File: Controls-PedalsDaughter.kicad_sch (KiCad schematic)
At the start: 3 parts, among them J3 PeripheralCANConnector, J5 PeripheralCANConnector, U2 PeripheralSOM

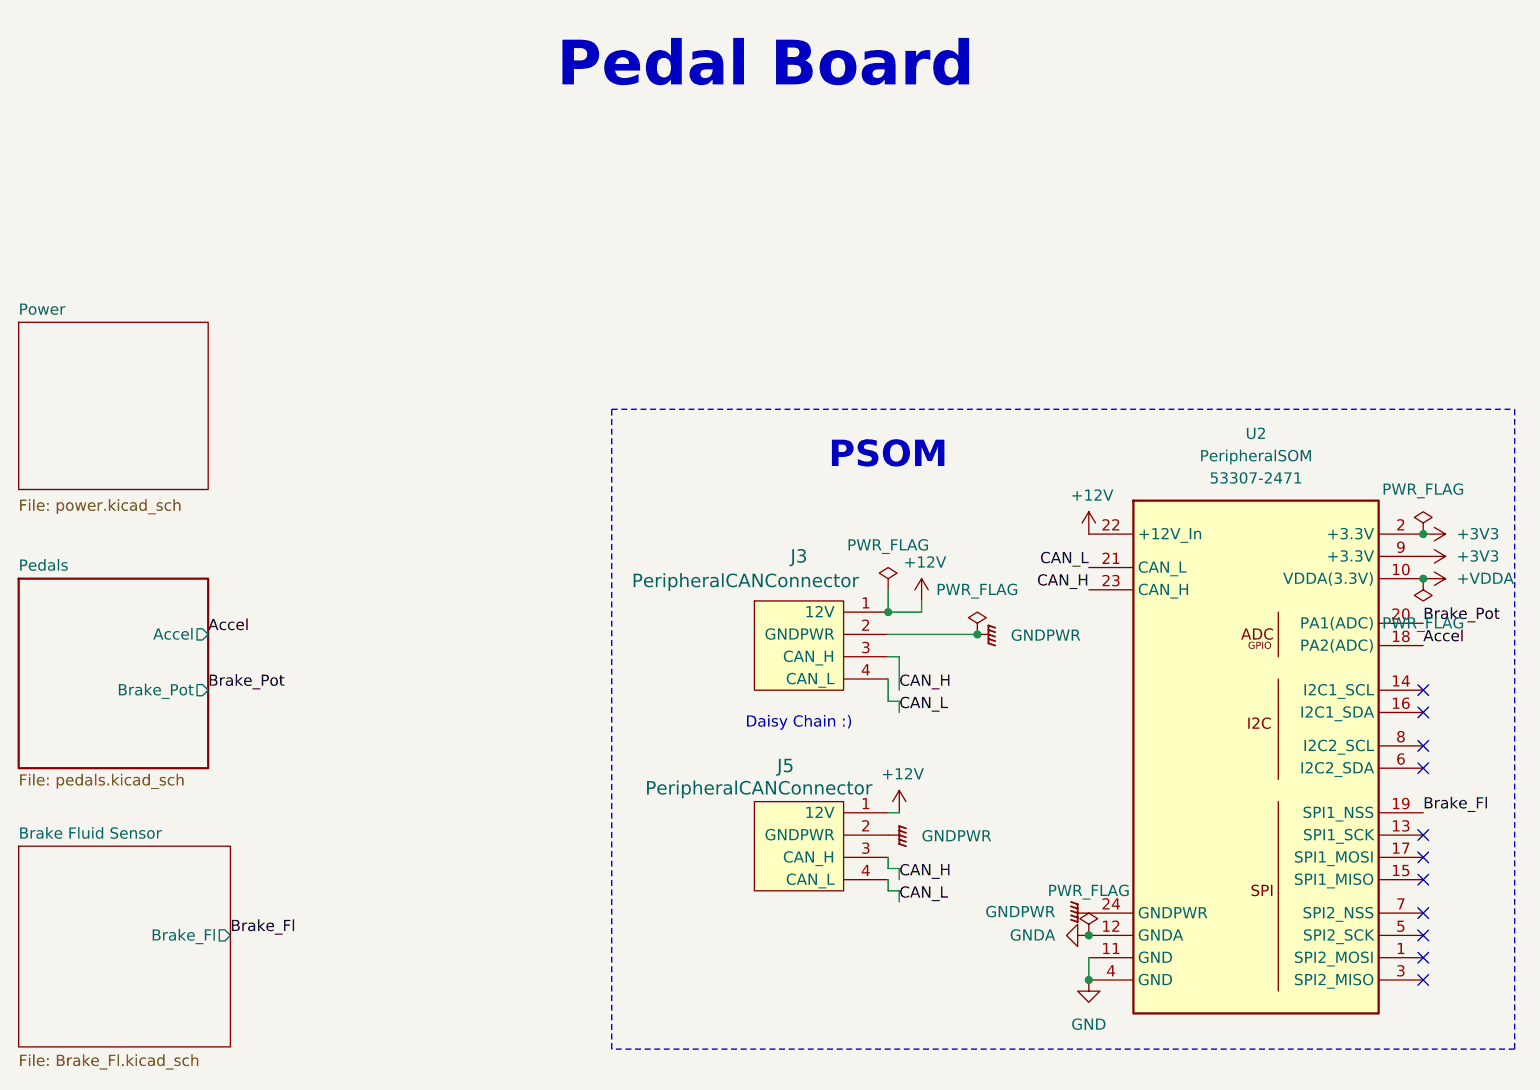
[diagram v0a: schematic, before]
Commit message: new constraints
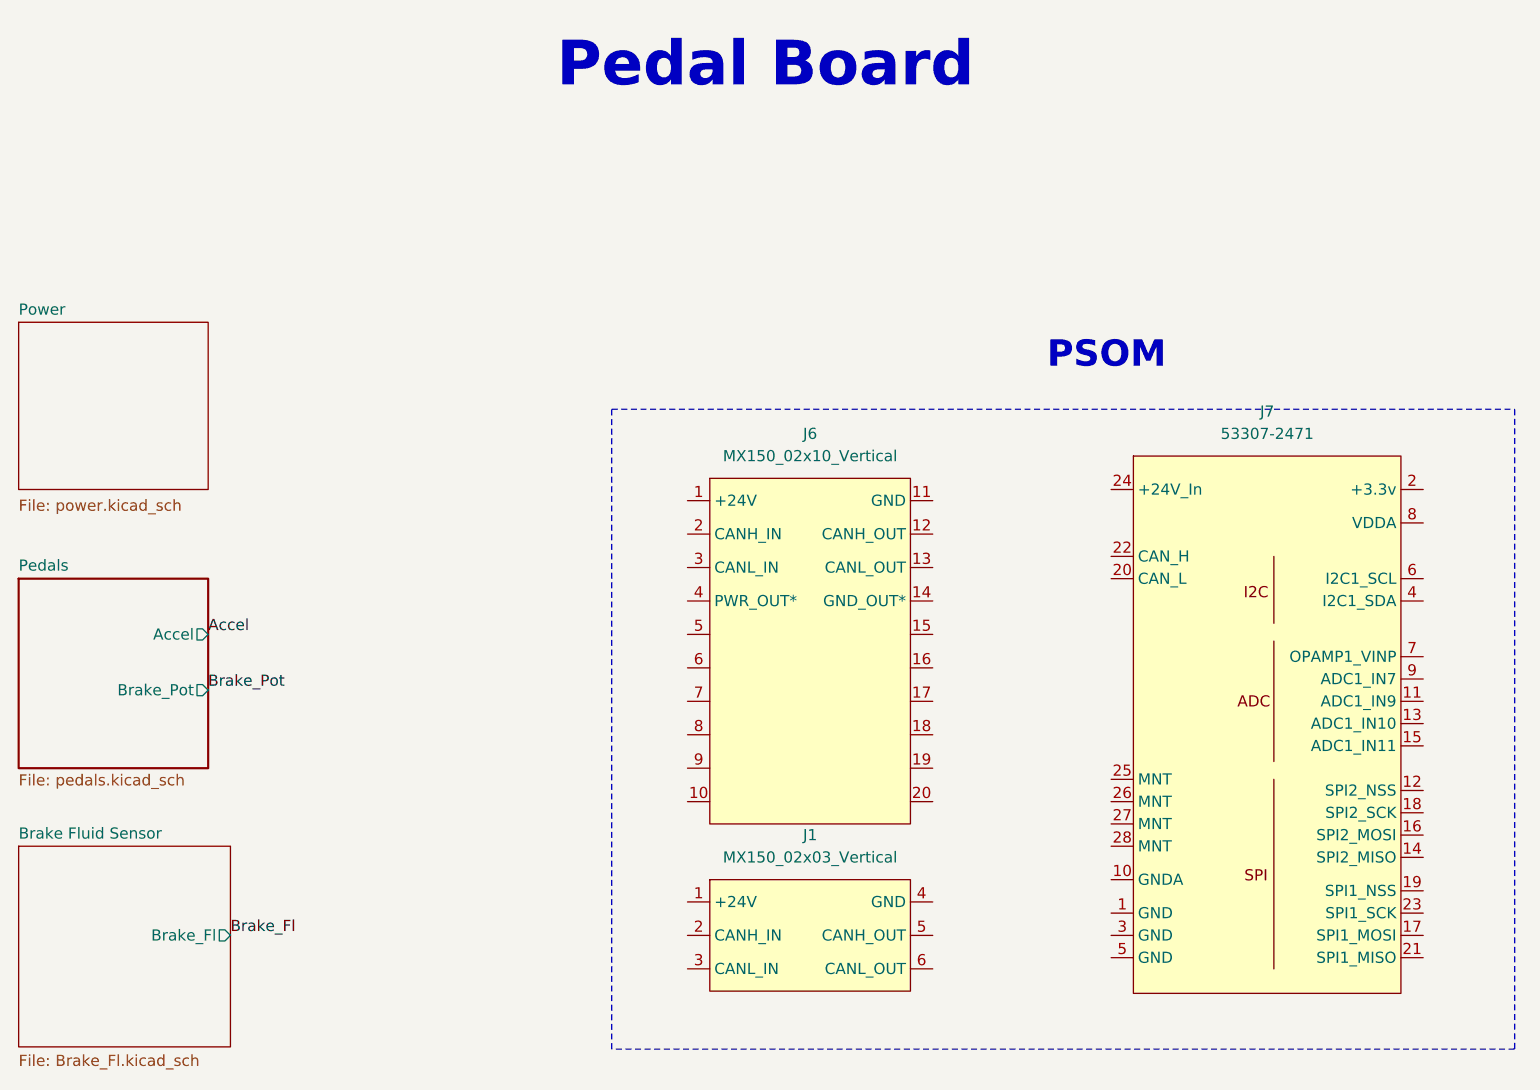
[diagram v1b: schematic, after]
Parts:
- removed J3, J5: PeripheralCANConnector, UTSVT_Connectors:Molex_MicroFit3.0_1x4xP3.00mm_PolarizingPeg_Vertical, symbol utsvt-connectors:PeripheralCANConnector
- removed U2: PeripheralSOM, UTSVT_Special:PeripheralSOM, symbol utsvt-misc:PeripheralSOM
- added J1: MX150_02x03_Vertical, UTSVT_Connectors:CONN06_0757575131_MOL, symbol utsvt_connectors:MX150_02x03_Vertical
- added J6: MX150_02x10_Vertical, UTSVT_Connectors:CONN_SD-75757-002_2X10_F16p09_MOL, symbol utsvt_connectors:MX150_02x10_Vertical
- added J7: 53307-2471, UTSVT_Connectors:PeripheralSOM, symbol utsvt_connectors:PeripheralSOMConnector
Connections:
- no-connect marks 11 -> 0
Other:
- note removed: "Daisy Chain :)"
